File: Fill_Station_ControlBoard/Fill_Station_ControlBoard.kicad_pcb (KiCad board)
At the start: 6 copper layers, 124 x 90 mm, 245 parts, among them IC1 TPS259573DSGR, J1 RJ45_Wuerth_7499010211A, J10 Micro_SD_Card_Det_Hirose_DM3AT, J12 Conn_02x05_Counter_Clockwise, J13 Screw_Terminal_2_P5.00mm, J14 Micro_SD_Card_Det_Hirose_DM3AT, J15 USB_C_Receptacle_USB2.0_14P, J16 DE9_Socket_MountingHoles, J18 Screw_Terminal_3_P3.50mm, J2 Ematch1, J6 Ematch2, J7 Screw_Terminal_3_P3.50mm, J8 Screw_Terminal_3_P3.50mm, J9 Screw_Terminal_6_P3.50mm, Q1 AO3400A, Q2 AO3400A, SW1 RESET, SW2 BOOT, U1 LAN8742A, U2 STM32H747IITx, U3 OKI-78SR-5_1.5-W36-C, U4 TPS62130, U6 TPS2116DRL, U7 USBLC6-2SC6, U8 ISOW1044, Y1 ASV-25.000MHz, Y2 ASV-32.768kHz, Y3 ASV-25.000MHz

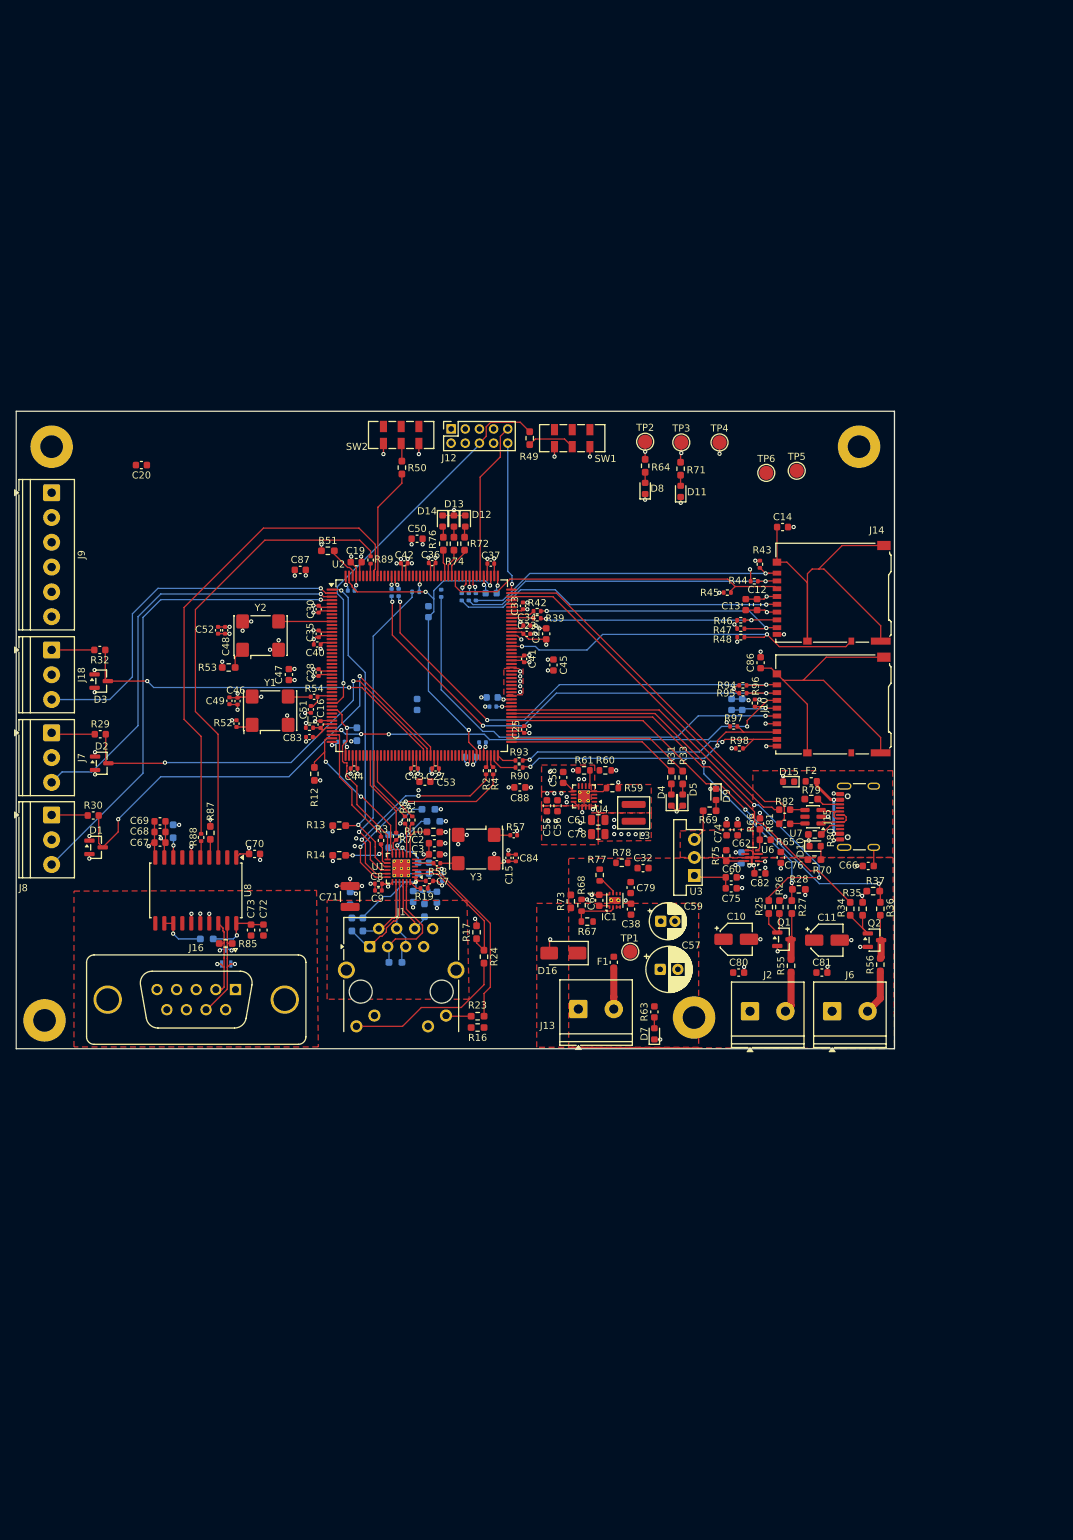
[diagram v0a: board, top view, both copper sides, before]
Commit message: Travail Layout
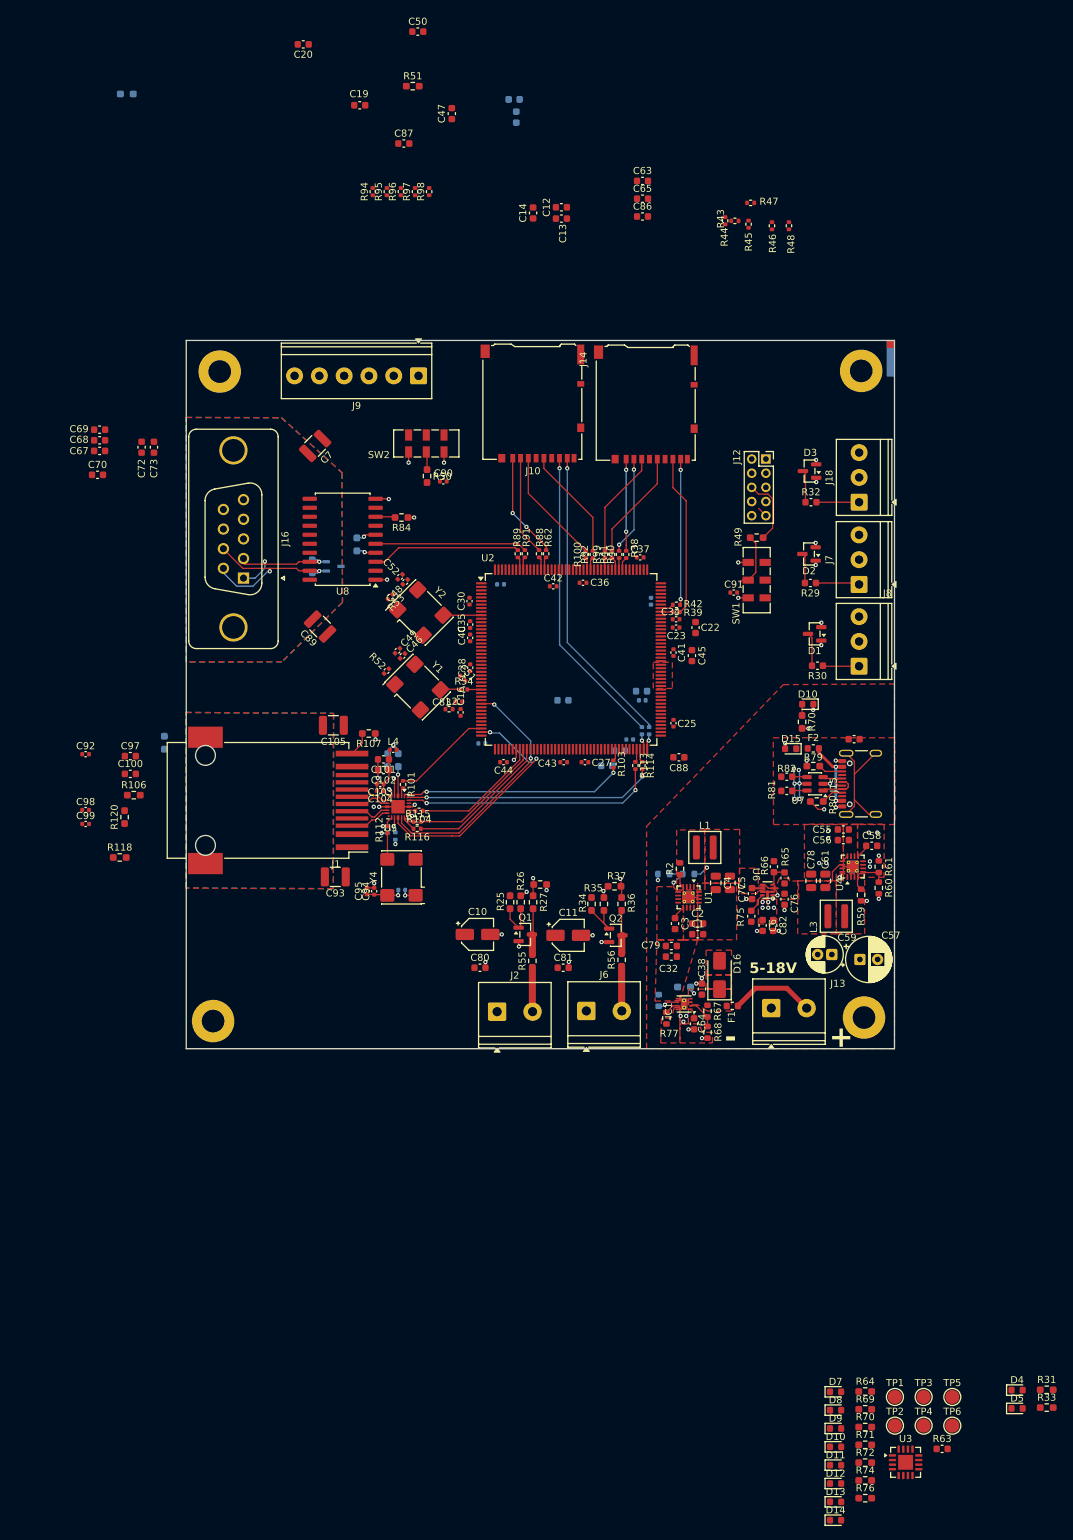
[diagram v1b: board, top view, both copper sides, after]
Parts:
- removed C15, C9: 100n, Capacitor_SMD:C_0402_1005Metric
- removed C60, C74: 100n, Capacitor_SMD:C_0603_1608Metric
- removed C62, C75: 22u, Capacitor_SMD:C_0603_1608Metric
- removed C71: 1000p - 2000V, Capacitor_SMD:C_1210_3225Metric
- removed C8: 100n, Resistor_SMD:R_0402_1005Metric
- removed C84: 10u, Capacitor_SMD:C_0402_1005Metric
- removed C85: *, Capacitor_SMD:C_0402_1005Metric
- removed R10, R11, R13, R14, R15, R16, R17, R5, R9: 10k, Resistor_SMD:R_0603_1608Metric_Pad0.98x0.95mm_HandSolder
- removed R12: 1k, Resistor_SMD:R_0603_1608Metric_Pad0.98x0.95mm_HandSolder
- removed R18, R20, R21, R22: 49.9, Resistor_SMD:R_0603_1608Metric_Pad0.98x0.95mm_HandSolder
- removed R19: 12.1k, Resistor_SMD:R_0402_1005Metric
- removed R23, R24: 270, Resistor_SMD:R_0603_1608Metric_Pad0.98x0.95mm_HandSolder
- removed R57: 10k, Capacitor_SMD:C_0402_1005Metric
- removed R58: 0, Capacitor_SMD:C_0402_1005Metric
- removed R6, R7, R8: 22, Resistor_SMD:R_0402_1005Metric
- removed R83: 1M, Resistor_SMD:R_0603_1608Metric_Pad0.98x0.95mm_HandSolder
- removed Y3: ASV-25.000MHz, Oscillator:Oscillator_SMD_Abracon_ASV-4Pin_7.0x5.1mm
- added C100: 10u, Capacitor_SMD:C_0603_1608Metric, F.Cu at (164.1, 139.2)
- added C101: 10u, Capacitor_SMD:C_0603_1608Metric, F.Cu at (199.8, 137.2)
- added C102: 1u, Capacitor_SMD:C_0603_1608Metric, F.Cu at (199.8, 138.7)
- added C103: 100n, Capacitor_SMD:C_0402_1005Metric, F.Cu at (199.4, 140.6)
- added C104: 10n, Capacitor_SMD:C_0402_1005Metric, F.Cu at (199.4, 141.6)
- added C105: 1000p - 2000V, Capacitor_SMD:C_1210_3225Metric, F.Cu at (192.8, 132.3)
- added C89: 1000p - 2000V, Capacitor_SMD:C_1210_3225Metric, F.Cu at (190.9, 118.4)
- added C90: 100n, Capacitor_SMD:C_0402_1005Metric, F.Cu at (208.3, 97.9)
- added C91: 100n, Capacitor_SMD:C_0402_1005Metric, F.Cu at (249.3, 113.6)
- added C92: 100n, Capacitor_SMD:C_0402_1005Metric, F.Cu at (157.8, 136.4)
- added C93: 1000p - 2000V, Capacitor_SMD:C_1210_3225Metric, F.Cu at (193.1, 153.7)
- added C94: 100n, Capacitor_SMD:C_0402_1005Metric, F.Cu at (198.5, 155.8)
- added C95: 10u, Capacitor_SMD:C_0402_1005Metric, F.Cu at (197.5, 155.7)
- added C96: *, Capacitor_SMD:C_0402_1005Metric, B.Cu at (200.4, 147.1)
- added C97: 1u, Capacitor_SMD:C_0603_1608Metric, F.Cu at (164.1, 136.7)
- added C98: 100n, Capacitor_SMD:C_0402_1005Metric, F.Cu at (157.8, 144.3)
- added C99: 10n, Capacitor_SMD:C_0402_1005Metric, F.Cu at (157.8, 146.3)
- added D10: LED, LED_SMD:LED_0603_1608Metric, F.Cu at (263.7, 234.2)
- added L4: L_Ferrite, Capacitor_SMD:C_0402_1005Metric, F.Cu at (201.2, 135.8)
- added R100: 22, Resistor_SMD:R_0402_1005Metric, F.Cu at (228.4, 108.2)
- added R101: 22, Resistor_SMD:R_0402_1005Metric, F.Cu at (202.6, 140.7)
- added R102: 6.49k, Resistor_SMD:R_0402_1005Metric, B.Cu at (201.5, 148.0)
- added R103: 22, Resistor_SMD:R_0402_1005Metric, F.Cu at (232.3, 137.8)
- added R104: 22, Resistor_SMD:R_0402_1005Metric, F.Cu at (204.9, 144.4)
- added R106: 1M, Resistor_SMD:R_0603_1608Metric_Pad0.98x0.95mm_HandSolder, F.Cu at (164.6, 142.2)
- added R107: 270, Resistor_SMD:R_0603_1608Metric_Pad0.98x0.95mm_HandSolder, F.Cu at (197.8, 133.5)
- added R111: 10k, Capacitor_SMD:C_0402_1005Metric, B.Cu at (202.4, 155.6)
- added R112: 0, Capacitor_SMD:C_0402_1005Metric, F.Cu at (200.4, 147.1)
- added R113: 22, Resistor_SMD:R_0402_1005Metric, F.Cu at (235.4, 138.0)
- added R114: 22, Resistor_SMD:R_0402_1005Metric, F.Cu at (236.4, 138.0)
- added R115: 22, Resistor_SMD:R_0402_1005Metric, F.Cu at (204.6, 145.9)
- added R116: 22, Resistor_SMD:R_0402_1005Metric, F.Cu at (204.6, 146.9)
- added R117: 10k, Resistor_SMD:R_0603_1608Metric_Pad0.98x0.95mm_HandSolder, B.Cu at (202.0, 137.3)
- added R118: 10k, Resistor_SMD:R_0603_1608Metric_Pad0.98x0.95mm_HandSolder, F.Cu at (162.6, 151.0)
- added R119: 10k, Resistor_SMD:R_0603_1608Metric_Pad0.98x0.95mm_HandSolder, B.Cu at (168.9, 134.8)
- added R120: 10k, Resistor_SMD:R_0603_1608Metric_Pad0.98x0.95mm_HandSolder, F.Cu at (163.3, 145.3)
- added R70: 1.5k, Resistor_SMD:R_0603_1608Metric_Pad0.98x0.95mm_HandSolder, F.Cu at (267.9, 231.4)
- added R99: 22, Resistor_SMD:R_0402_1005Metric, F.Cu at (231.1, 108.2)
- added U5: DP83825I, Package_DFN_QFN:Texas_RMQ0024A_WQFN-24-1EP_3x3mm_P0.4mm_EP1.9x1.9mm, F.Cu at (201.9, 143.8)
- added Y4: ASV-25.000MHz, Oscillator:Oscillator_SMD_Abracon_ASV-4Pin_7.0x5.1mm, F.Cu at (202.4, 153.8)
- C1: value 1u -> 10u; moved to F.Cu
- C2: value 1uF -> 0.1u
- C3: value 470pF -> 3.3n
- C33, C53, R73, R78, R85, R87, R90, R93: moved to B.Cu
- C4: value 100n -> 22u; footprint Capacitor_SMD:C_0603_1608Metric -> Capacitor_SMD:C_0805_2012Metric; moved to F.Cu
- C5: value 10u -> 22u; footprint Capacitor_SMD:C_0603_1608Metric -> Capacitor_SMD:C_0805_2012Metric; moved to F.Cu
- C6, C63, C65, C77, R38, R40, R41, R62, R84, R91, R92: moved to F.Cu
- C7: value 100n -> 1000p - 2000V; footprint Resistor_SMD:R_0402_1005Metric -> Capacitor_SMD:C_1210_3225Metric
- J1: value RJ45_Wuerth_7499010211A -> RJ45_Wuerth_74980111211; footprint Connector_RJ:RJ45_Wuerth_7499010211A_Horizontal -> Connector_RJ:RJ45_Wuerth_74980111211_Horizontal
- L1: value L_Ferrite -> 2.2u; footprint Capacitor_SMD:C_0402_1005Metric -> Inductor_SMD:L_Coilcraft_XAL4020-XXX; moved to F.Cu
- R1: value 22 -> 10k; footprint Resistor_SMD:R_0402_1005Metric -> Resistor_SMD:R_0603_1608Metric_Pad0.98x0.95mm_HandSolder; moved to B.Cu
- R2: value 22 -> 100k; footprint Resistor_SMD:R_0402_1005Metric -> Resistor_SMD:R_0603_1608Metric
- R3: value 22 -> 100k; footprint Resistor_SMD:R_0402_1005Metric -> Resistor_SMD:R_0603_1608Metric; moved to B.Cu
- R4: value 22 -> 316k; footprint Resistor_SMD:R_0402_1005Metric -> Resistor_SMD:R_0603_1608Metric; moved to B.Cu
- R53: footprint Resistor_SMD:R_0603_1608Metric_Pad0.98x0.95mm_HandSolder -> Capacitor_SMD:C_0402_1005Metric
- U1: value LAN8742A -> TPS62130; footprint Package_DFN_QFN:VQFN-24-1EP_4x4mm_P0.5mm_EP2.5x2.5mm_ThermalVias -> Package_DFN_QFN:VQFN-16-1EP_3x3mm_P0.5mm_EP1.68x1.68mm_ThermalVias
- U3: value OKI-78SR-5_1.5-W36-C -> INA3221; footprint Converter_DCDC:Converter_DCDC_Murata_OKI-78SR_Vertical -> Package_DFN_QFN:Texas_RGV0016A_VQFN-16-1EP_4x4mm_P0.65mm_EP2.1x2.1mm
- moved D14 151.6 mm to (263.7, 244.6), turned to 0 degrees
- moved D13 148.6 mm to (263.7, 242.0), turned to 0 degrees
- moved R76 147.3 mm to (267.9, 241.5), turned to 0 degrees
- moved D12 145.6 mm to (263.7, 239.4), turned to 0 degrees
- moved R74 144.4 mm to (267.9, 238.9), turned to 0 degrees
- moved TP2 143.3 mm to (272.1, 231.2)
- moved TP4 141.8 mm to (276.1, 231.2)
- moved R72 141.5 mm to (267.9, 236.4), turned to 0 degrees
- moved R71 140.3 mm to (267.9, 233.9), turned to 0 degrees
- moved D11 139.2 mm to (263.7, 236.8), turned to 0 degrees
- moved TP3 139.0 mm to (276.1, 227.2)
- moved TP6 137.1 mm to (280.2, 231.2)
- moved R64 134.3 mm to (267.9, 226.4), turned to 0 degrees
- moved D8 132.9 mm to (263.7, 229.0), turned to 0 degrees
- moved TP5 132.6 mm to (280.2, 227.2)
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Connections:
- C1 pad 1: 3V3 -> 12.8V
- C2 pad 1: Net-(U1-VDDCR) -> 12.8V
- C3 pad 1: Net-(U1-VDDCR) -> Net-(U1-SS/TR)
- C4 pad 1: 3V3 -> 3V3_Bat
- C5 pad 1: 3V3 -> 3V3_Bat
- C55 pad 1: 5V -> 5V_USB
- C56 pad 1: 5V -> 5V_USB
- C6 pad 1: 3V3A_Eth -> 3V3
- C61 pad 1: 3V3 -> 3V3_USB
- C7 pad 1: 3V3A_Eth -> GND
- C7 pad 2: GND -> CHASSIS_CAN
- C76 pad 1: 5V_USB -> 3V3_USB
- C77 pad 1: 5V_BAT -> 3V3_Bat
- C78 pad 1: 3V3 -> 3V3_USB
- C82 pad 1: 5V -> 3V3
- J1 pad 1: /Ethernet/TX_P -> unconnected-(J1-Pad1)
- J1 pad 10: GND -> CHASSIS_ETH
- J1 pad 11: GND -> /Ethernet/LED0
- J1 pad 2: /Ethernet/TX_N -> unconnected-(J1-Pad2)
- J1 pad 3: /Ethernet/RX_P -> /Ethernet/TX_P
- J1 pad 4: 3V3A_Eth -> Net-(J1-RCT)
- J1 pad 5: 3V3A_Eth -> /Ethernet/TX_N
- J1 pad 6: /Ethernet/RX_N -> /Ethernet/RX_P
- J1 pad 7: unconnected-(J1-NC-Pad7) -> Net-(J1-RCT)
- J1 pad 8: CHASSIS_ETH -> /Ethernet/RX_N
- J1 pad 9: Net-(J1-Pad9) -> unconnected-(J1-NC-Pad9)
- J10 pad 10: unconnected-(J10-DET_A-Pad10) -> /MCU/SD2.DET
- J10 pad 3: /MCU/SD2.CMD -> Net-(J10-CMD)
- J12 pad 8: /MCU/SWO -> unconnected-(J12-Pin_8-Pad8)
- J14 pad 3: /MCU/SD1.CMD -> Net-(J14-CMD)
- J16 pad 1: unconnected-(J16-Pad1) -> /CAN FD/CAN_N
- J16 pad 6: unconnected-(J16-Pad6) -> /CAN FD/CAN_P
- J16 pad 8: unconnected-(J16-Pad8) -> CHASSIS_CAN
- L1 pad 1: 3V3 -> /Alimentation/3V3_SW
- L1 pad 2: 3V3A_Eth -> 3V3_Bat
- L3 pad 1: /Alimentation/3V3_SW -> /Alimentation/3V3_SW_USB
- L3 pad 2: 3V3 -> 3V3_USB
- R1 pad 1: /Ethernet/Eth.RXD1 -> 3V3
- R1 pad 2: Net-(U1-RXD1/MODE1) -> /Ethernet/Eth.RST
- R2 pad 1: /Ethernet/Eth.TXD0 -> Net-(U1-PG)
- R2 pad 2: /Ethernet/TXD_P -> 3V3_Bat
- R3 pad 1: /Ethernet/Eth.REFCLKO -> Net-(U1-FB)
- R3 pad 2: Net-(U1-~{INT}/REFCLKO) -> 3V3_Bat
- R4 pad 1: /Ethernet/Eth.TXD1 -> GND
- R4 pad 2: /Ethernet/TXD_N -> Net-(U1-FB)
- R45 pad 2: /MCU/SD1.CMD -> Net-(J14-CMD)
- R59 pad 2: 3V3 -> 3V3_USB
- R60 pad 2: 3V3 -> 3V3_USB
- R65 pad 2: 5V_USB -> 3V3_USB
- R72 pad 2: /Alimentation/LED1 -> /Monitor/LED1
- R74 pad 2: /Alimentation/LED2 -> /Monitor/LED2
- R75 pad 2: 5V_BAT -> 3V3
- R76 pad 2: /Alimentation/LED3 -> /Monitor/LED3
- R78 pad 2: 3V3 -> 12.8V
- R96 pad 2: /MCU/SD2.CMD -> Net-(J10-CMD)
- U1 pad 1: 3V3A_Eth -> /Alimentation/3V3_SW
- U1 pad 10: Net-(U1-RXER/PHYAD0) -> 12.8V
- U1 pad 11: Net-(U1-CRS_DV/MODE2) -> 12.8V
- U1 pad 12: /Ethernet/Eth.MDIO -> 12.8V
- U1 pad 13: /Ethernet/Eth.MDC -> 12.8V
- U1 pad 14: Net-(U1-~{INT}/REFCLKO) -> 3V3_Bat
- U1 pad 15: /Ethernet/Eth.RST -> GND
- U1 pad 16: Net-(U1-TXEN) -> GND
- U1 pad 17: /Ethernet/TXD_P -> GND
- U1 pad 2: /Ethernet/LED2 -> /Alimentation/3V3_SW
- U1 pad 3: /Ethernet/LED1 -> /Alimentation/3V3_SW
- U1 pad 4: unconnected-(U1-XTAL2-Pad4) -> Net-(U1-PG)
- U1 pad 5: /Ethernet/Eth_Clock_25Mhz -> Net-(U1-FB)
- U1 pad 6: Net-(U1-VDDCR) -> GND
- U1 pad 7: Net-(U1-RXD1/MODE1) -> GND
- U1 pad 8: Net-(U1-RXD0/MODE0) -> GND
- U1 pad 9: 3V3 -> Net-(U1-SS/TR)
- U2 pad 1: /Ethernet/Eth.RST -> unconnected-(U2-PE2-Pad1)
- U2 pad 146: /Alimentation/LED1 -> /MCU/LED1
- U2 pad 147: /Alimentation/LED2 -> /MCU/LED2
- U2 pad 148: /Alimentation/LED3 -> /MCU/LED3
- U2 pad 150: unconnected-(U2-PD7-Pad150) -> /MCU/SD2.CMD
- U2 pad 155: /Ethernet/Eth.TXEN -> unconnected-(U2-PG11-Pad155)
- U2 pad 170: /MCU/CAN.FAULT -> unconnected-(U2-PE0-Pad170)
- U2 pad 41: /MCU/SD2.CMD -> unconnected-(U2-PA0-Pad41)
- U2 pad 51: unconnected-(U2-PA6-Pad51) -> /Ethernet/Eth.RST
- U2 pad 53: /Ethernet/Eth.RXD0 -> /Ethernet/Eth.RXD_P
- U2 pad 54: /Ethernet/Eth.RXD1 -> /Ethernet/Eth.RXD_N
- U2 pad 79: unconnected-(U2-PB11-Pad79) -> Net-(U2-PB11)
- U2 pad 85: /Ethernet/Eth.TXD0 -> Net-(U2-PB12)
- U2 pad 86: /Ethernet/Eth.TXD1 -> Net-(U2-PB13)
- U3 pad 1: 12.8V -> unconnected-(U3-IN-3-Pad1)
- U3 pad 2: GND -> unconnected-(U3-IN+3-Pad2)
- U3 pad 3: 5V_BAT -> unconnected-(U3-GND-Pad3)
- U4 pad 1: /Alimentation/3V3_SW -> /Alimentation/3V3_SW_USB
- U4 pad 10: 5V -> 5V_USB
- U4 pad 11: 5V -> 5V_USB
- U4 pad 12: 5V -> 5V_USB
- U4 pad 13: 5V -> 5V_USB
- U4 pad 14: 3V3 -> 3V3_USB
- U4 pad 2: /Alimentation/3V3_SW -> /Alimentation/3V3_SW_USB
- U4 pad 3: /Alimentation/3V3_SW -> /Alimentation/3V3_SW_USB
- U6 pad 2: 5V -> 3V3
- U6 pad 3: 5V_USB -> 3V3_USB
- U6 pad 5: 5V_USB -> 3V3_USB
- U6 pad 6: 5V_BAT -> 3V3_Bat
- U6 pad 7: 5V -> 3V3
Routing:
- net GND: track 162.2 -> 50.3 mm, vias 124 -> 54
- net 3V3: track 114.8 -> 21.5 mm, vias 71 -> 16
- net /CAN FD/CAN.RXD: track 70.1 -> 1.84 mm
- net /Control/Heater3: track 68.0 -> 0.00 mm, vias 1 -> 0
- net /MCU/SD2.CMD: track 67.1 -> 1.71 mm, vias 4 -> 0
- net /Control/Servo.Signal3: track 69.9 -> 4.73 mm, vias 2 -> 0
- net /Control/E-match1: track 63.0 -> 0.49 mm, vias 2 -> 0
- net /Control/E-match2_Det: track 64.2 -> 2.77 mm, vias 2 -> 1
- net /Control/Heater2: track 59.8 -> 0.00 mm, vias 1 -> 0
- net /Control/E-match2: track 59.5 -> 0.00 mm
- net /Control/Servo.Signal2: track 60.6 -> 4.25 mm, vias 2 -> 0
- net Net-(J10-DAT3/CD): track 69.9 -> 14.1 mm, vias 3 -> 0
- net Net-(J14-SHIELD): track 54.9 -> 0.00 mm
- net /MCU/USBC.DP: track 53.8 -> 0.00 mm
- net Net-(J10-DAT2): track 68.5 -> 14.9 mm, vias 3 -> 2
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- added copper zone on F.Cu, net /Alimentation/3V3_SW_USB
- added copper zone on F.Cu, net 3V3_Bat
- added copper zone on F.Cu, net 3V3_USB
- added copper zone on B.Cu, net CHASSIS_CAN
- added copper zone on B.Cu, net CHASSIS_ETH
- removed copper zone on F.Cu, net 5V
- removed copper zone on F.Cu, net 5V_BAT
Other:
- board size 124 x 90 mm -> 100 x 100 mm
- board text added: "+"
- board text added: "-"
- board text added: "5-18V"
- board text added: "Pas de fil icite"
- board text added: "Stitch osc"
- board text removed: "3V3"
- board text removed: "5V"
- board text removed: "GND1"
- board text removed: "GND2"
